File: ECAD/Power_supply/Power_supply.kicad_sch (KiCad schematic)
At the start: 52 parts, among them J1 Barrel_Jack_Switch, J2 Conn_01x06, Q1 DMP3037LSS-13, SW1 SW_Push_DPDT, U1 LM317_TO-220, U2 LM317_TO-220, U3 LM317_TO-220

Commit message: Added heatsink 3D model.
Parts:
- HS1, HS2, HS3: footprint Heatsink:Heatsink_Fischer_SK104-STC-STIC_35x13mm_2xDrill2.5mm -> Heatsink_custom:Heatsink_Fischer_SK104-STC-STIC_35x13mm_2xDrill2.5mm
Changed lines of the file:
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@@
 			)
 		)
-		(property "Footprint" "Heatsink:Heatsink_Fischer_SK104-STC-STIC_35x13mm_2xDrill2.5mm"
+		(property "Footprint" "Heatsink_custom:Heatsink_Fischer_SK104-STC-STIC_35x13mm_2xDrill2.5mm"
 			(at 101.9048 95.25 0)
 			(effects
@@
 			)
 		)
-		(property "Footprint" "Heatsink:Heatsink_Fischer_SK104-STC-STIC_35x13mm_2xDrill2.5mm"
+		(property "Footprint" "Heatsink_custom:Heatsink_Fischer_SK104-STC-STIC_35x13mm_2xDrill2.5mm"
 			(at 178.1048 95.25 0)
 			(effects
@@
 			)
 		)
-		(property "Footprint" "Heatsink:Heatsink_Fischer_SK104-STC-STIC_35x13mm_2xDrill2.5mm"
+		(property "Footprint" "Heatsink_custom:Heatsink_Fischer_SK104-STC-STIC_35x13mm_2xDrill2.5mm"
 			(at 101.9048 151.13 0)
 			(effects

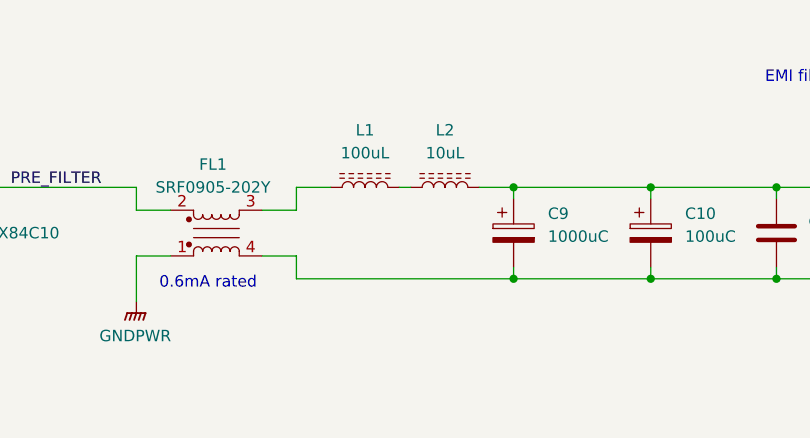
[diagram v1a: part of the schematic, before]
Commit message: Progressed PCB.
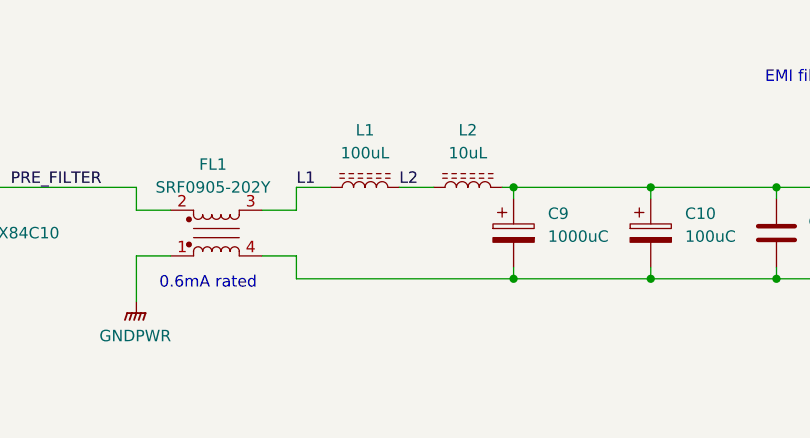
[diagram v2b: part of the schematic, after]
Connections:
- net L2: now reaches L1.2, L2.1
- net L1: now reaches FL1.3, L1.1
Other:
- moved on the sheet: L2
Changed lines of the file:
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@@
 	(wire
 		(pts
-			(xy 154.94 33.02) (xy 158.75 33.02)
+			(xy 157.48 33.02) (xy 158.75 33.02)
 		)
 		(stroke
@@
 	(wire
 		(pts
-			(xy 146.05 33.02) (xy 147.32 33.02)
+			(xy 146.05 33.02) (xy 149.86 33.02)
 		)
 		(stroke
@@
 	(label "PRE_FILTER"
 		(at 102.87 33.02 0)
+		(effects
+			(font
+				(size 1.27 1.27)
+			)
+			(justify left bottom)
+		)
+	)
+	(label "L1"
+		(at 134.62 33.02 0)
+		(effects
+			(font
+				(size 1.27 1.27)
+			)
+			(justify left bottom)
+		)
+	)
+	(label "L2"
+		(at 146.05 33.02 0)
 		(effects
 			(font
@@
 	(symbol
 		(lib_id "Device:L_Ferrite")
-		(at 151.13 33.02 90)
+		(at 153.67 33.02 90)
 		(unit 1)
 		(exclude_from_sim no)
@@
 		(fields_autoplaced yes)
 		(property "Reference" "L2"
-			(at 151.13 26.67 90)
+			(at 153.67 26.67 90)
 			(effects
 				(font
@@
 		)
 		(property "Value" "10uL"
-			(at 151.13 29.21 90)
+			(at 153.67 29.21 90)
 			(effects
 				(font
@@
 		)
 		(property "Footprint" "Inductor_SMD:L_Taiyo-Yuden_NR-30xx"
-			(at 151.13 33.02 0)
+			(at 153.67 33.02 0)
 			(effects
 				(font
@@
 		)
 		(property "Datasheet" "https://datasheet.lcsc.com/lcsc/2304140030_Taiyo-Yuden-NR3015T100M_C87168.pdf"
-			(at 151.13 33.02 0)
+			(at 153.67 33.02 0)
 			(effects
 				(font
@@
 		)
 		(property "Description" ""
-			(at 151.13 33.02 0)
+			(at 153.67 33.02 0)
 			(effects
 				(font
@@
 		)
 		(property "MPN" "NR3015T100M"
-			(at 151.13 33.02 0)
+			(at 153.67 33.02 0)
 			(effects
 				(font
@@
 		)
 		(property "Status" "OK"
-			(at 151.13 33.02 0)
-			(effects
-				(font
+			(at 153.67 33.02 0)
+			(effects
+				(font
